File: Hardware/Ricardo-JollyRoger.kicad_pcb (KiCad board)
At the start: 4 copper layers, 45.1 x 35.1 mm, 87 parts, among them J1 RBUS, J2 USB_C_Receptacle_USB2.0, J3 Conn_01x08_Pin, U1 ESP32-S3, U2 SN65HVD230, U3 LM66200DRLR, U4 MAX77827AEFD+T, U5 SC4215ASTRT, U7 LM66200DRLR, Y1 R940000171

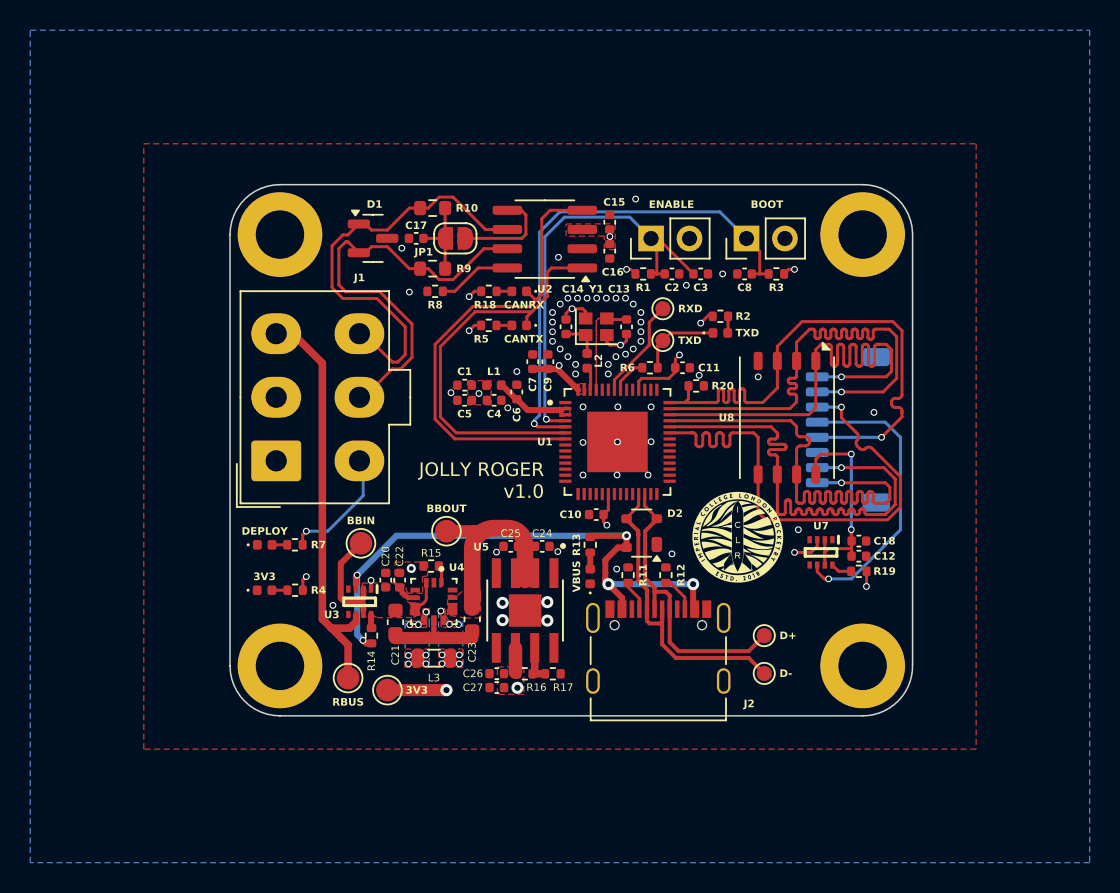
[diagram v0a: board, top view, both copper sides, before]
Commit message: Increase board size
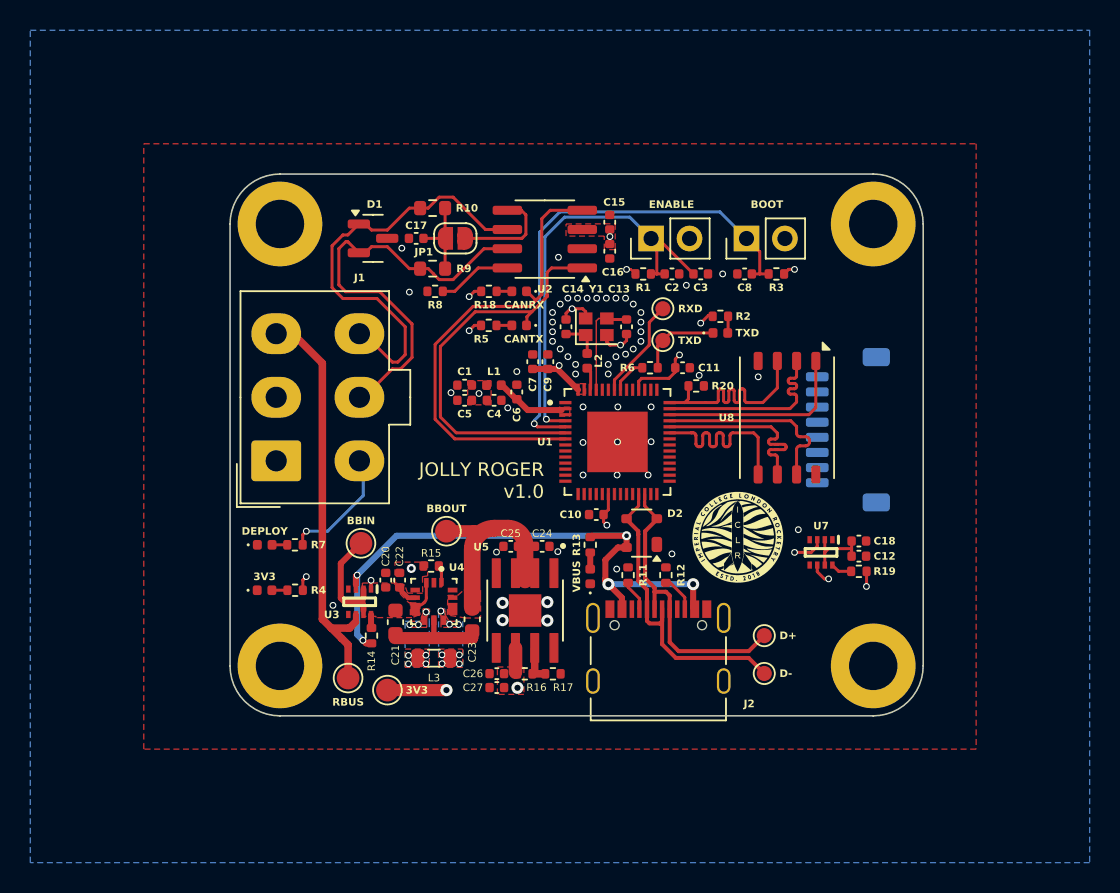
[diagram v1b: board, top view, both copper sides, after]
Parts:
- moved H2 0.99 mm to (121.6, 48.4)
- moved H1 0.70 mm to (82.4, 48.4)
- moved H3 0.70 mm to (121.6, 77.6)
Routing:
- net /NAND_CLK: track 38.1 -> 15.1 mm, vias 1 -> 0
- net /NAND_CMD: track 35.8 -> 12.9 mm, vias 1 -> 0
- net /NAND_SD2: track 35.8 -> 12.9 mm, vias 1 -> 0
- net /NAND_SD3: track 35.8 -> 13.0 mm, vias 1 -> 0
- net /NAND_SD1: track 35.8 -> 13.0 mm, vias 1 -> 0
- net /NAND_SD0: track 35.7 -> 13.0 mm, vias 1 -> 0
- net /HEADER_3V3: track 19.5 -> 1.38 mm
- net /NAND_3V3: track 13.8 -> 4.58 mm, vias 2 -> 0
- net GND: vias 61 -> 59
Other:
- board size 45.1 x 35.1 mm -> 45.8 x 35.8 mm
